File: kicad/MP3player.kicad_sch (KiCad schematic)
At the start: 6 parts

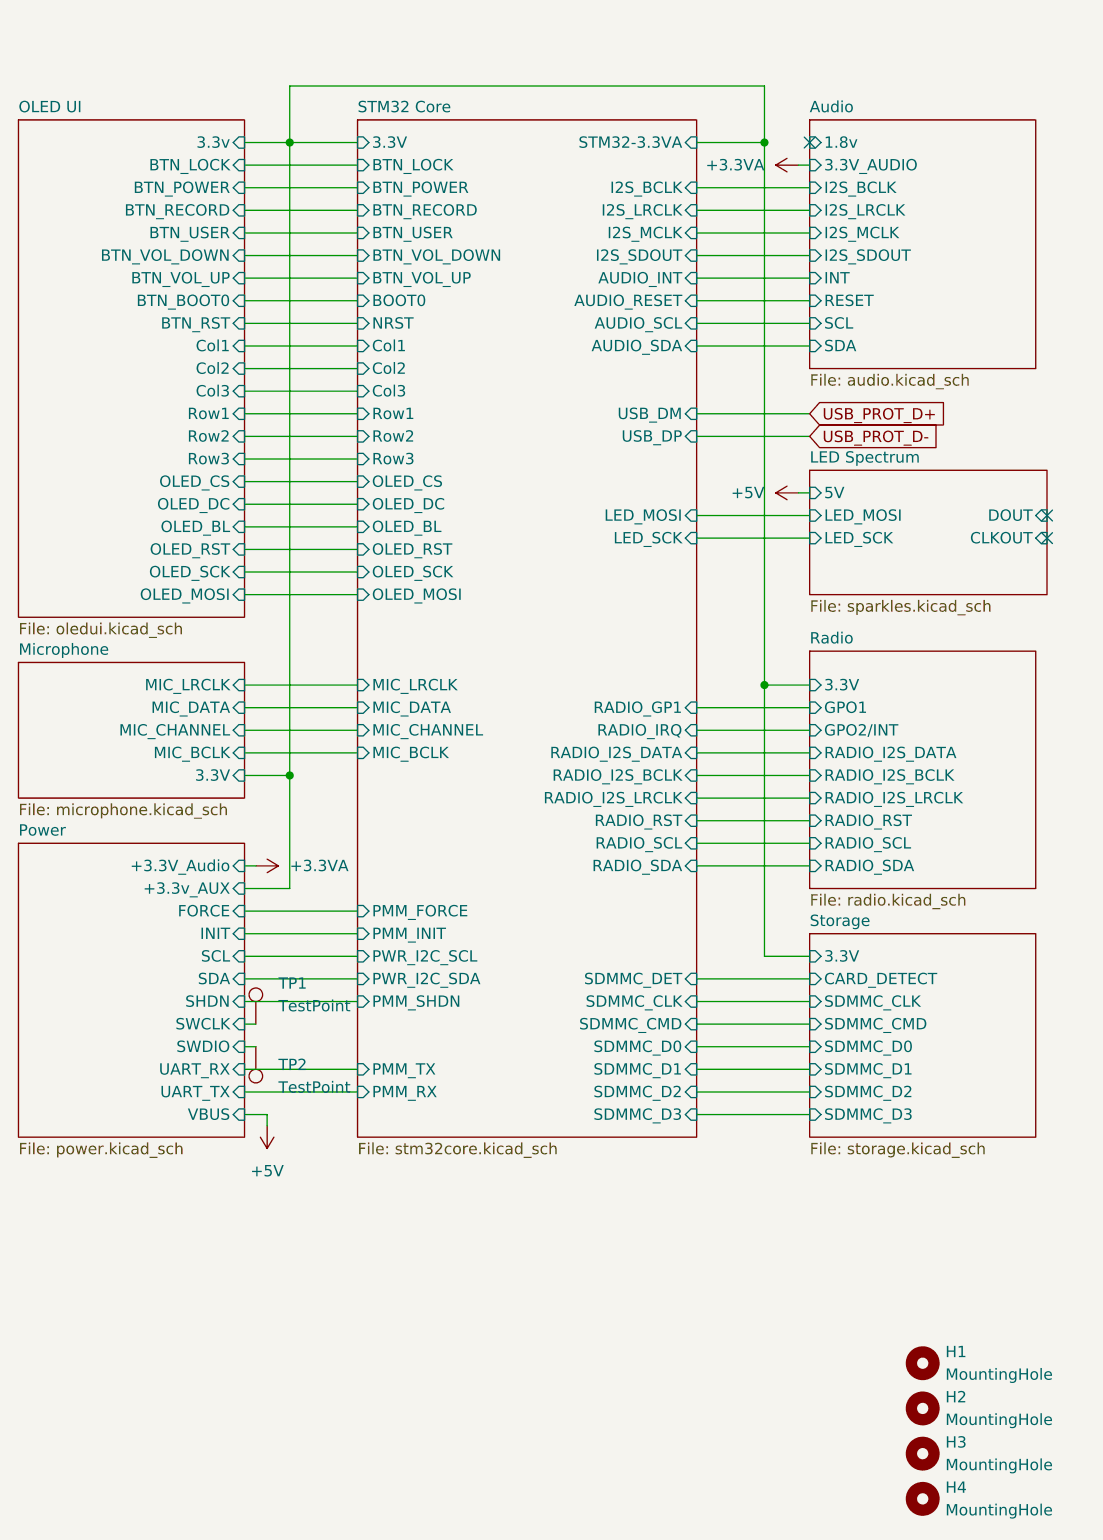
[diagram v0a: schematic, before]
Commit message: general changes
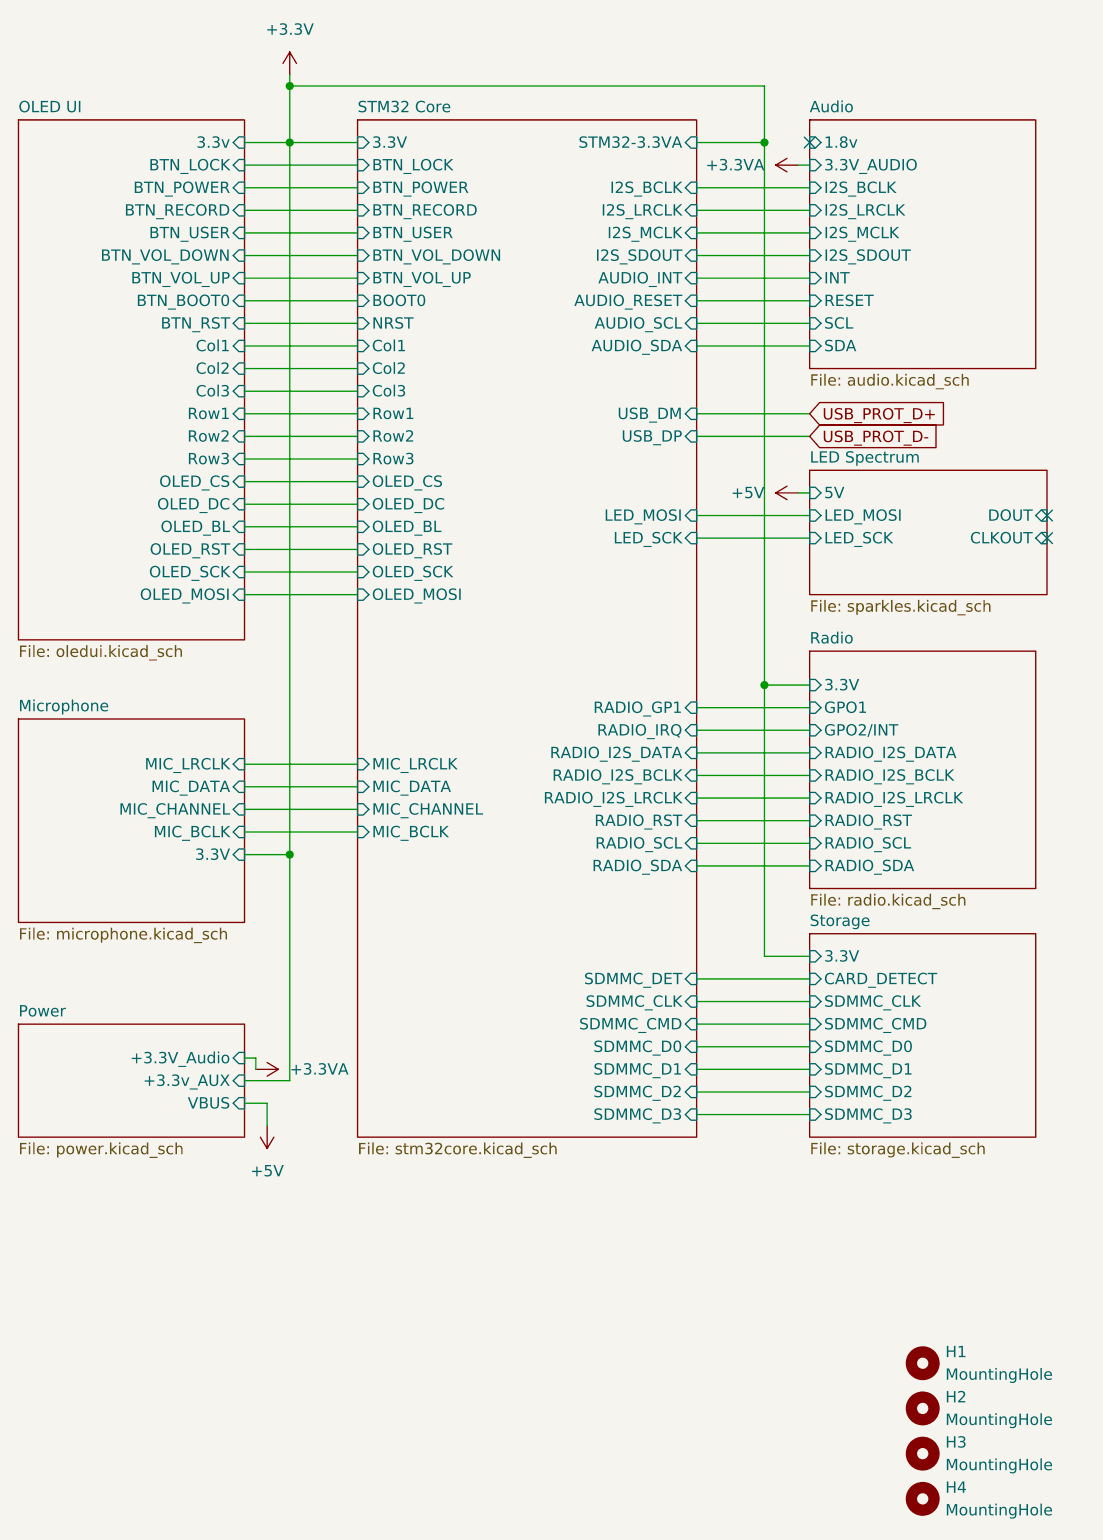
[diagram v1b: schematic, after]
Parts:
- removed TP1, TP2: TestPoint, symbol Connector:TestPoint
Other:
- sheet Power ports: added none; removed FORCE, INIT, SCL, SDA, SHDN, SWCLK, SWDIO, UART_RX, UART_TX
- sheet STM32 Core ports: added none; removed PMM_FORCE, PMM_INIT, PMM_RX, PMM_SHDN, PMM_TX, PWR_I2C_SCL, PWR_I2C_SDA
